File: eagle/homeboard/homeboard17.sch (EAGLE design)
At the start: 128 parts, among them IC1 XCF02S, IC2 25LC080SN, IC3 ATMEGA32U2-TQFP, Q5 BC848SMD, Q6 BC848SMD, Q7 BC848SMD, Q8 BC848SMD, T1 BSS138, T2 BC848, T3 BSS138, T4 BC848, U1 XC3S400TQ144, X1 SCART-CLIP, X6 MINI-USB_4P-85-32004-10X, X7 DC21MMX, X8 STEREOJACK

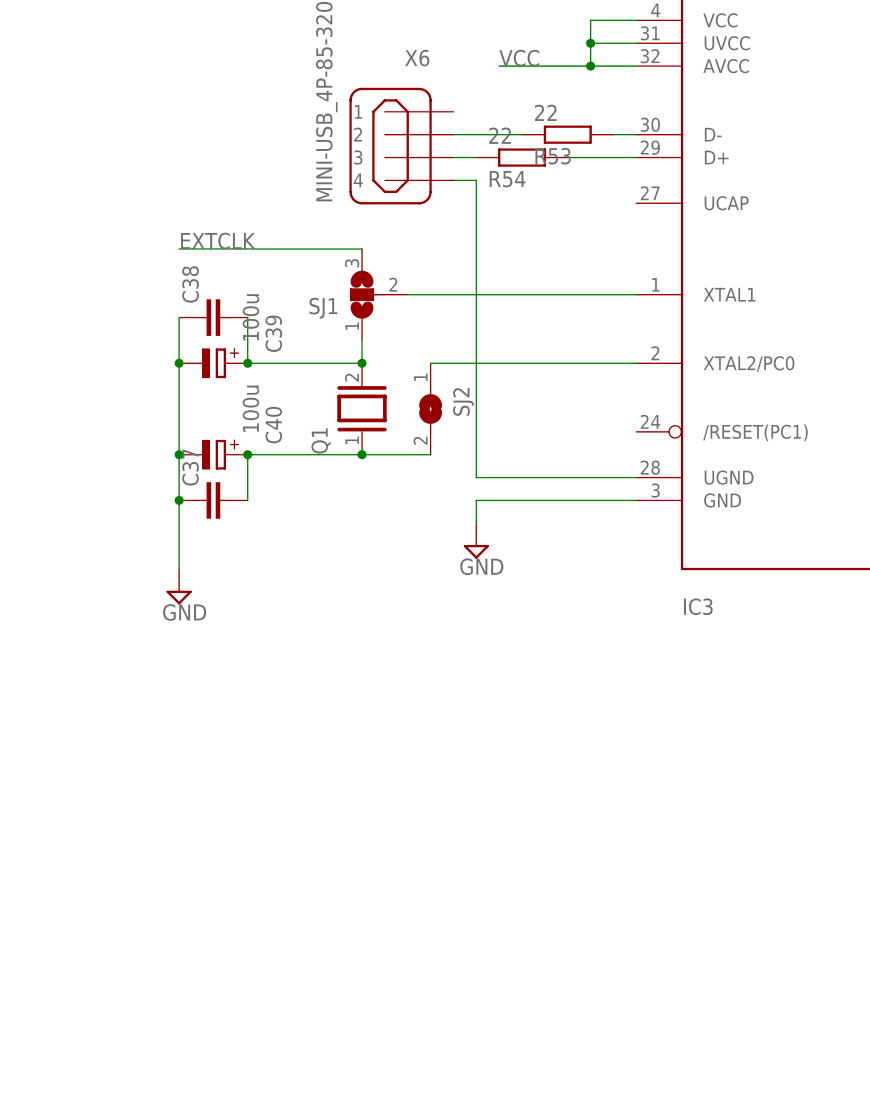
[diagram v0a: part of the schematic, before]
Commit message: mah
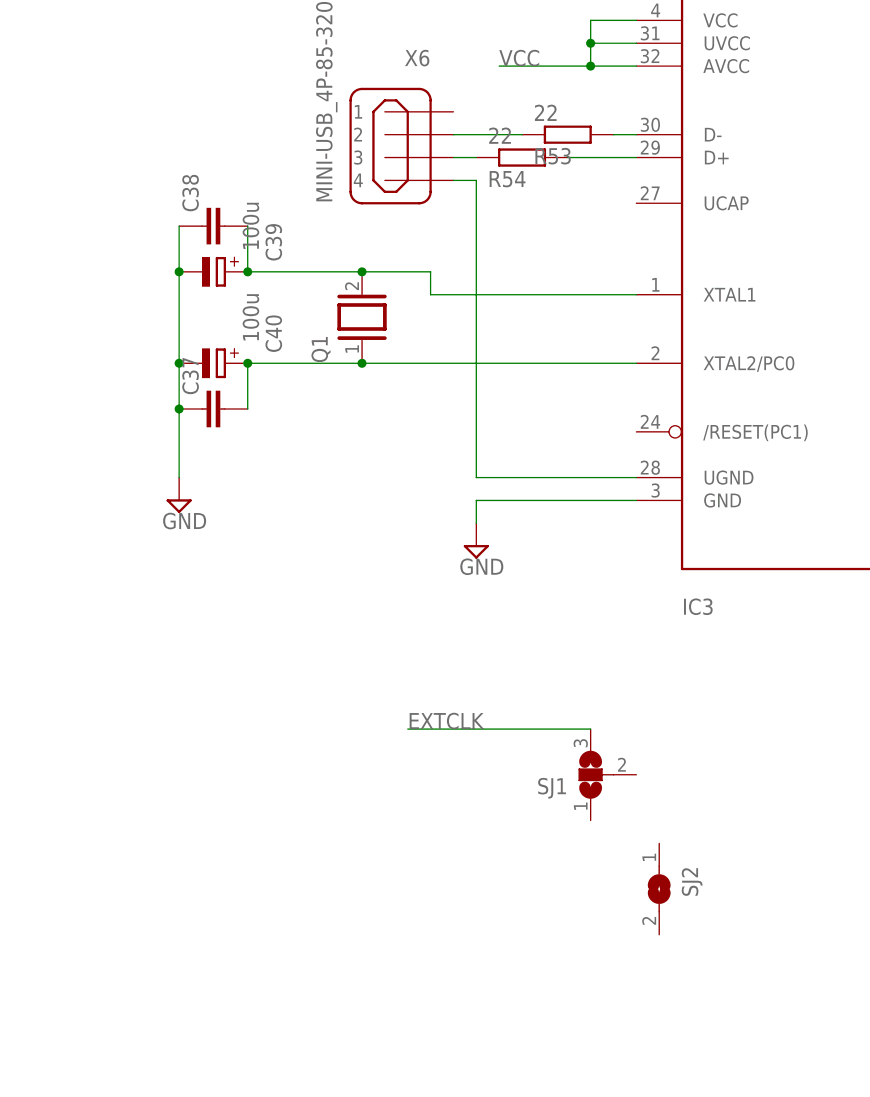
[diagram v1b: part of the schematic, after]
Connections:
- removed net N$10: IC3.XTAL2/PC0, SJ2.1
- removed net N$9: IC3.XTAL1, SJ1.2
- net N$12: now also IC3.XTAL2/PC0; no longer SJ2.2
- net N$14: now also IC3.XTAL1; no longer SJ1.1
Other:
- moved on the sheet: C37, C38, C39, C40, Q1, SJ1, SJ2
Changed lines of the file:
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@@
 <instance part="SV1" gate="1" x="43.18" y="-58.42" rot="R270"/>
 <instance part="SUPPLY19" gate="GND" x="109.22" y="83.82"/>
-<instance part="Q1" gate="G$1" x="353.06" y="91.44" rot="R90"/>
-<instance part="SJ1" gate="G$1" x="353.06" y="104.14" rot="R180"/>
-<instance part="SJ2" gate="1" x="360.68" y="91.44" rot="R270"/>
-<instance part="C37" gate="G$1" x="335.28" y="81.28" rot="R90"/>
-<instance part="C38" gate="G$1" x="335.28" y="101.6" rot="R90"/>
-<instance part="SUPPLY20" gate="GND" x="332.74" y="71.12"/>
-<instance part="C39" gate="G$1" x="337.82" y="96.52" smashed="yes" rot="R270">
+<instance part="Q1" gate="G$1" x="353.06" y="101.6" rot="R90"/>
+<instance part="SJ1" gate="G$1" x="378.46" y="50.8" rot="R180"/>
+<instance part="SJ2" gate="1" x="386.08" y="38.1" rot="R270"/>
+<instance part="C37" gate="G$1" x="335.28" y="91.44" rot="R90"/>
+<instance part="C38" gate="G$1" x="335.28" y="111.76" rot="R90"/>
+<instance part="SUPPLY20" gate="GND" x="332.74" y="81.28"/>
+<instance part="C39" gate="G$1" x="337.82" y="106.68" smashed="yes" rot="R270">
+<attribute name="NAME" x="342.3666" y="112.141" size="1.778" layer="95" rot="R270"/>
+<attribute name="VALUE" x="339.8266" y="114.554" size="1.778" layer="96" rot="R270"/>
+</instance>
+<instance part="C40" gate="G$1" x="337.82" y="96.52" smashed="yes" rot="R270">
 <attribute name="NAME" x="342.3666" y="101.981" size="1.778" layer="95" rot="R270"/>
 <attribute name="VALUE" x="339.8266" y="104.394" size="1.778" layer="96" rot="R270"/>
-</instance>
-<instance part="C40" gate="G$1" x="337.82" y="86.36" smashed="yes" rot="R270">
-<attribute name="NAME" x="342.3666" y="91.821" size="1.778" layer="95" rot="R270"/>
-<attribute name="VALUE" x="339.8266" y="94.234" size="1.778" layer="96" rot="R270"/>
 </instance>
 <instance part="PWR_HDR" gate="A" x="-297.18" y="50.8" rot="R90"/>
@@
 <pinref part="C38" gate="G$1" pin="1"/>
 <pinref part="C39" gate="G$1" pin="-"/>
-<wire x1="332.74" y1="101.6" x2="332.74" y2="96.52" width="0.1524" layer="91"/>
+<wire x1="332.74" y1="111.76" x2="332.74" y2="106.68" width="0.1524" layer="91"/>
 <pinref part="C40" gate="G$1" pin="-"/>
-<wire x1="332.74" y1="96.52" x2="332.74" y2="86.36" width="0.1524" layer="91"/>
+<wire x1="332.74" y1="106.68" x2="332.74" y2="96.52" width="0.1524" layer="91"/>
+<junction x="332.74" y="106.68"/>
+<pinref part="C37" gate="G$1" pin="1"/>
+<wire x1="332.74" y1="96.52" x2="332.74" y2="91.44" width="0.1524" layer="91"/>
 <junction x="332.74" y="96.52"/>
-<pinref part="C37" gate="G$1" pin="1"/>
-<wire x1="332.74" y1="86.36" x2="332.74" y2="81.28" width="0.1524" layer="91"/>
-<junction x="332.74" y="86.36"/>
 <pinref part="SUPPLY20" gate="GND" pin="GND"/>
-<wire x1="332.74" y1="73.66" x2="332.74" y2="81.28" width="0.1524" layer="91"/>
-<junction x="332.74" y="81.28"/>
+<wire x1="332.74" y1="83.82" x2="332.74" y2="91.44" width="0.1524" layer="91"/>
+<junction x="332.74" y="91.44"/>
 </segment>
 <segment>
@@
 </segment>
 </net>
-<net name="N$9" class="0">
-<segment>
-<pinref part="IC3" gate="G$1" pin="XTAL1"/>
-<pinref part="SJ1" gate="G$1" pin="2"/>
-<wire x1="383.54" y1="104.14" x2="358.14" y2="104.14" width="0.1524" layer="91"/>
-</segment>
-</net>
-<net name="N$10" class="0">
-<segment>
-<pinref part="IC3" gate="G$1" pin="XTAL2/PC0"/>
-<pinref part="SJ2" gate="1" pin="1"/>
-<wire x1="383.54" y1="96.52" x2="360.68" y2="96.52" width="0.1524" layer="91"/>
-</segment>
-</net>
 <net name="EXTCLK" class="0">
 <segment>
 <pinref part="SJ1" gate="G$1" pin="3"/>
-<wire x1="353.06" y1="109.22" x2="332.74" y2="109.22" width="0.1524" layer="91"/>
-<label x="332.74" y="109.22" size="1.778" layer="95"/>
+<wire x1="378.46" y1="55.88" x2="358.14" y2="55.88" width="0.1524" layer="91"/>
+<label x="358.14" y="55.88" size="1.778" layer="95"/>
 </segment>
 </net>
@@
 <pinref part="C37" gate="G$1" pin="2"/>
 <pinref part="C40" gate="G$1" pin="+"/>
-<wire x1="340.36" y1="81.28" x2="340.36" y2="86.36" width="0.1524" layer="91"/>
-<pinref part="SJ2" gate="1" pin="2"/>
+<wire x1="340.36" y1="91.44" x2="340.36" y2="96.52" width="0.1524" layer="91"/>
 <pinref part="Q1" gate="G$1" pin="1"/>
-<wire x1="360.68" y1="86.36" x2="353.06" y2="86.36" width="0.1524" layer="91"/>
-<wire x1="340.36" y1="86.36" x2="353.06" y2="86.36" width="0.1524" layer="91"/>
-<junction x="340.36" y="86.36"/>
-<junction x="353.06" y="86.36"/>
+<wire x1="340.36" y1="96.52" x2="353.06" y2="96.52" width="0.1524" layer="91"/>
+<junction x="340.36" y="96.52"/>
+<pinref part="IC3" gate="G$1" pin="XTAL2/PC0"/>
+<wire x1="383.54" y1="96.52" x2="353.06" y2="96.52" width="0.1524" layer="91"/>
+<junction x="353.06" y="96.52"/>
 </segment>
 </net>
@@
 <pinref part="C38" gate="G$1" pin="2"/>
 <pinref part="C39" gate="G$1" pin="+"/>
-<pinref part="SJ1" gate="G$1" pin="1"/>
 <pinref part="Q1" gate="G$1" pin="2"/>
-<wire x1="353.06" y1="96.52" x2="353.06" y2="99.06" width="0.1524" layer="91"/>
-<junction x="353.06" y="96.52"/>
-<wire x1="353.06" y1="96.52" x2="340.36" y2="96.52" width="0.1524" layer="91"/>
-<wire x1="340.36" y1="96.52" x2="340.36" y2="101.6" width="0.1524" layer="91"/>
-<junction x="340.36" y="96.52"/>
-</segment>
-</net>
+<wire x1="353.06" y1="106.68" x2="340.36" y2="106.68" width="0.1524" layer="91"/>
+<wire x1="340.36" y1="106.68" x2="340.36" y2="111.76" width="0.1524" layer="91"/>
+<junction x="340.36" y="106.68"/>
+<pinref part="IC3" gate="G$1" pin="XTAL1"/>
+<wire x1="383.54" y1="104.14" x2="360.68" y2="104.14" width="0.1524" layer="91"/>
+<wire x1="360.68" y1="104.14" x2="360.68" y2="106.68" width="0.1524" layer="91"/>
+<wire x1="360.68" y1="106.68" x2="353.06" y2="106.68" width="0.1524" layer="91"/>
+<junction x="353.06" y="106.68"/>
+</segment>
+</net>
